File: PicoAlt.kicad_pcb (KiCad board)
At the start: 2 copper layers, 20.3 x 57.8 mm, 37 parts, among them J2 USB_B, J3 Conn_01x04, J4 Conn_01x20, J5 Conn_01x20, SW1 SW_Push, SW2 SW_Push, U1 AMS1117-3.3, U2 W25Q128JVSIQ, U3 RP2040, Y1 12 MHz

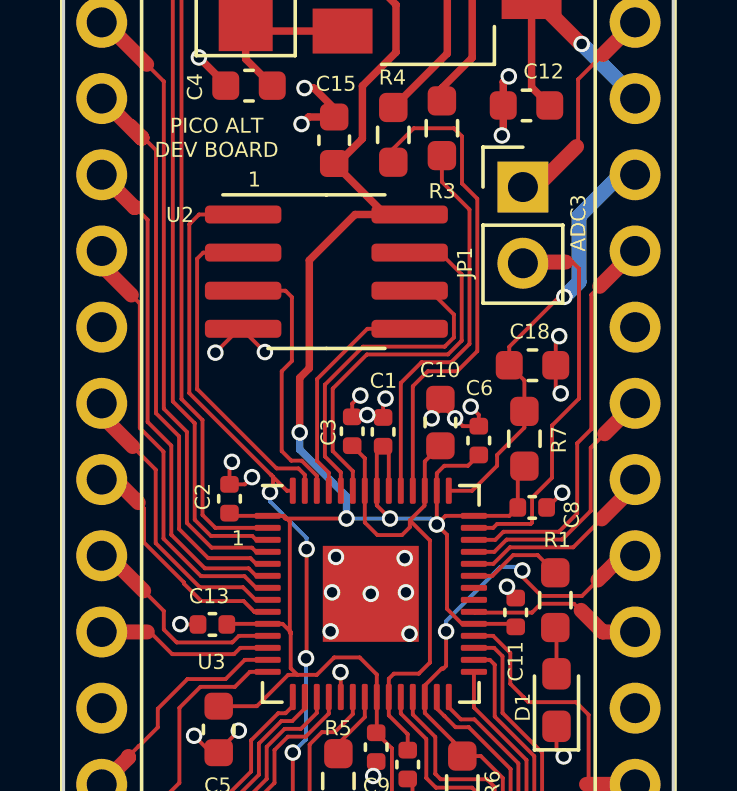
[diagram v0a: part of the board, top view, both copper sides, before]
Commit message: JLCPCB #2
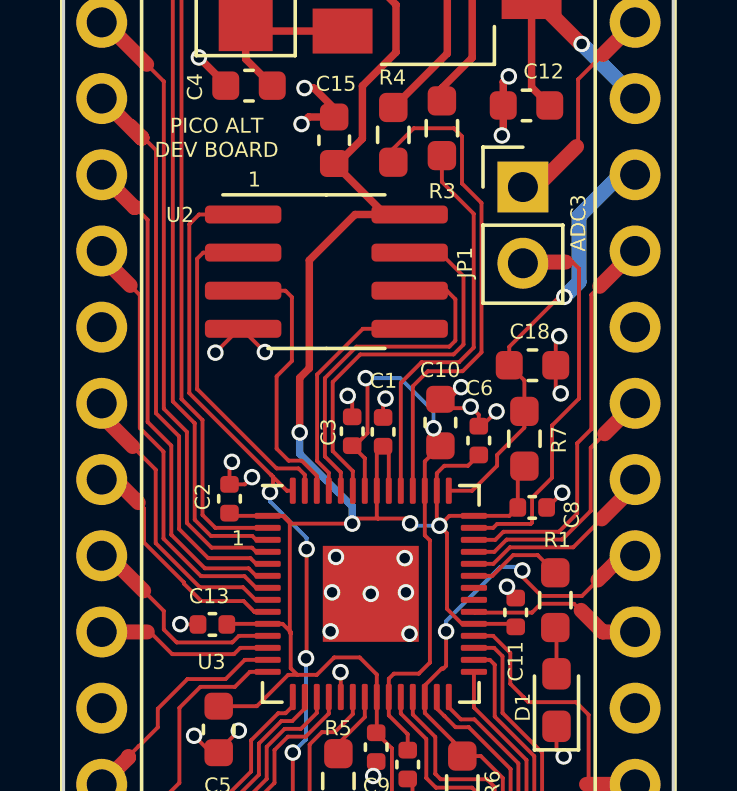
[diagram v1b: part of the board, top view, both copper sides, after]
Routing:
- net +1V1: track 16.9 -> 19.9 mm, vias 0 -> 2
- net GND: track 48.5 -> 47.9 mm, vias 42 -> 41
